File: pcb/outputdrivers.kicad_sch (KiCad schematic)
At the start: 24 parts, among them IC1 DRV8874QPWPRQ1, J7 CP/PE, J7 RF, Q1 BC846, Q2 NCV8402xST, Q3 NCV8402xST, Q4 DTA143Z, Q7 DTC114E, Q8 DTC114E, Q9 DTC114E, U7 74HCT04

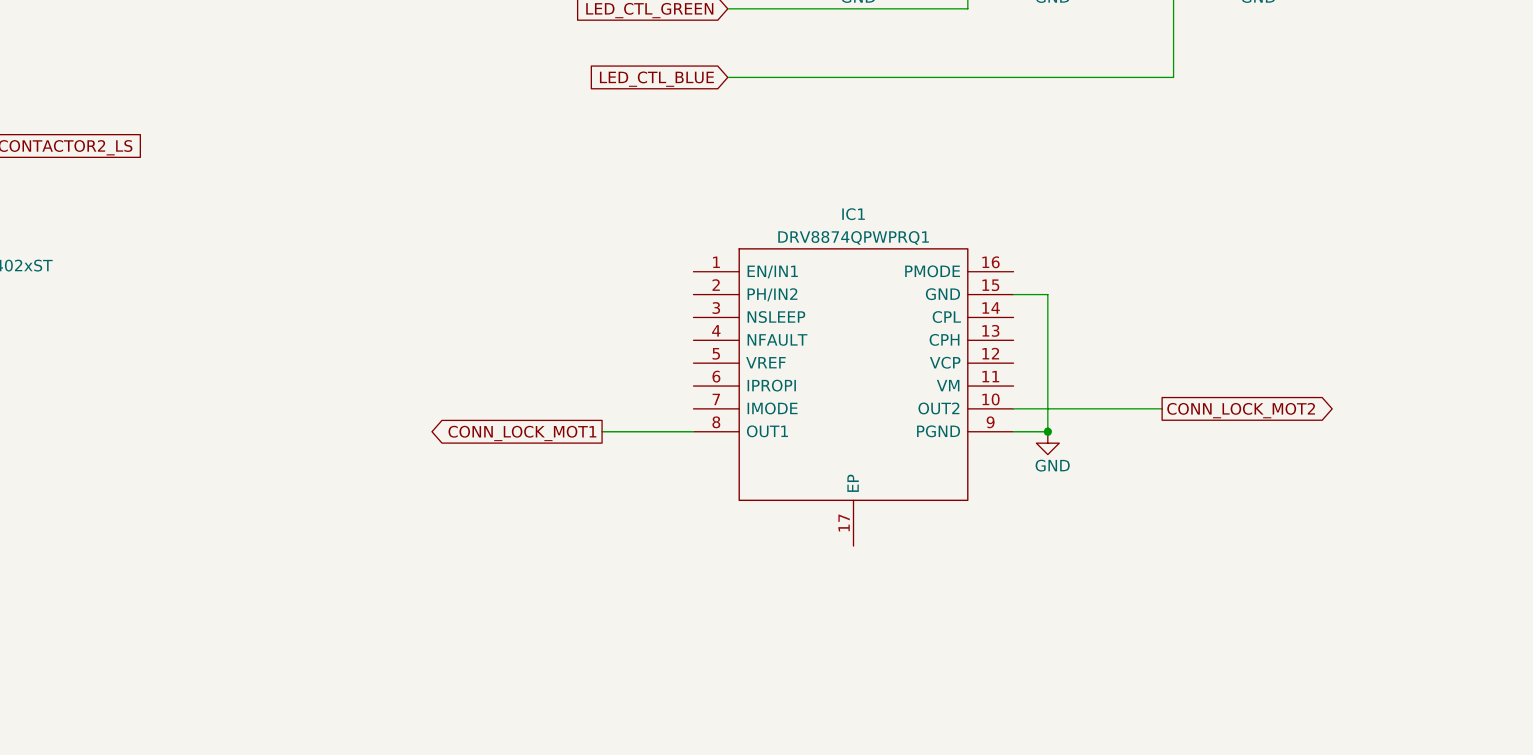
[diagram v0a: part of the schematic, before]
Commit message: wired the drv8874. Added spare holes. Flash connector larger holes
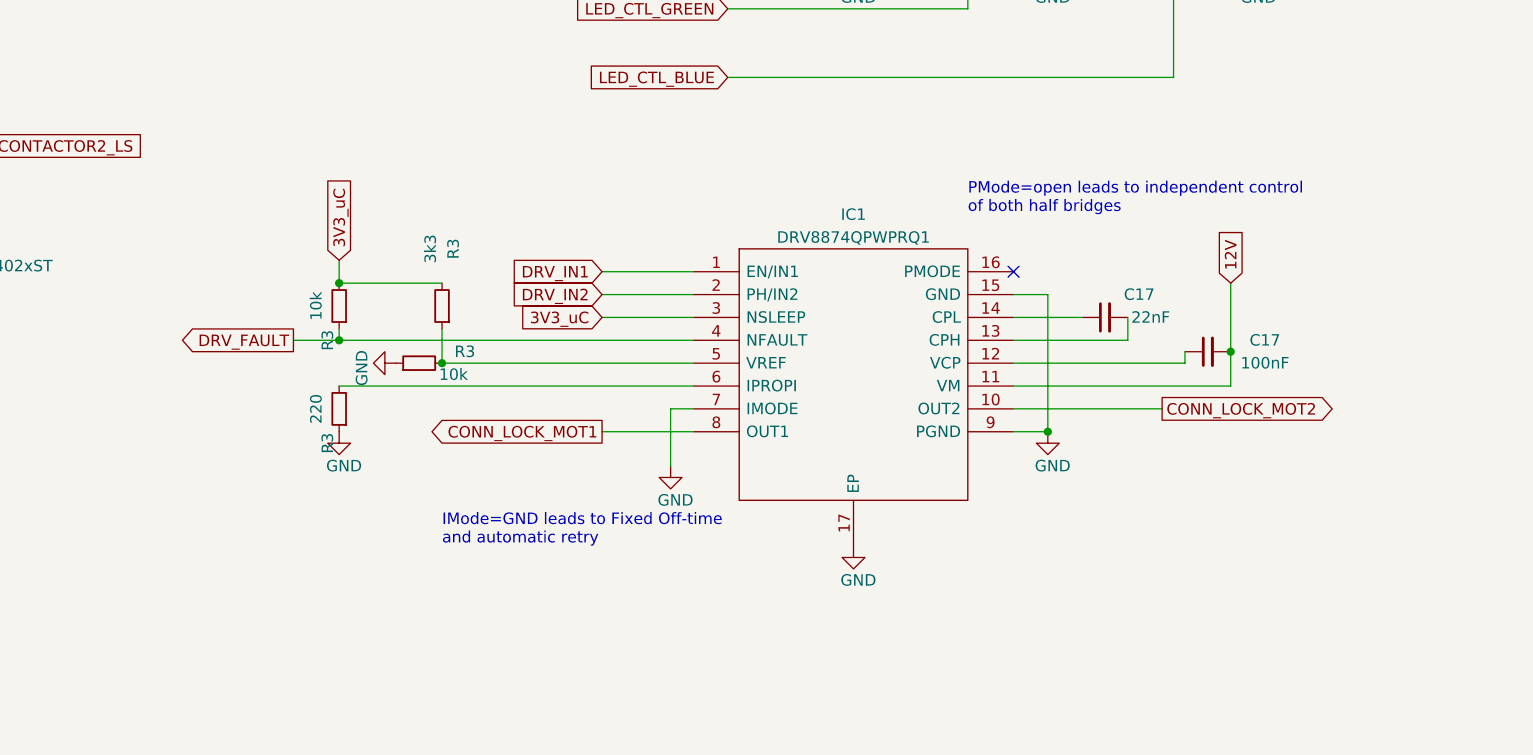
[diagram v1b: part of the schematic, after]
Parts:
- added C17: 100nF, Capacitor_SMD:C_0805_2012Metric_Pad1.18x1.45mm_HandSolder, symbol Device:C_Small
- added C17: 22nF, Capacitor_SMD:C_0805_2012Metric_Pad1.18x1.45mm_HandSolder, symbol Device:C_Small
- added R3: 3k3, Resistor_SMD:R_1206_3216Metric_Pad1.30x1.75mm_HandSolder, symbol Device:R_Small
- added R3: 220, Resistor_SMD:R_1206_3216Metric_Pad1.30x1.75mm_HandSolder, symbol Device:R_Small
- added R3 (x2): 10k, Resistor_SMD:R_1206_3216Metric_Pad1.30x1.75mm_HandSolder, symbol Device:R_Small
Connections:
- net GND: now also IC1.17 (EP), IC1.7 (IMODE), R3.1, R3.1
- net DRV_IN1: now reaches IC1.1 (EN/IN1)
- net 12V: now reaches IC1.11 (VM)
- net 12V: now also C17.2
- net at IC1.12 (VCP): now also C17.1
- net at IC1.13 (CPH): now also C17.2
- net at IC1.14 (CPL): now also C17.1
- net DRV_IN2: now reaches IC1.2 (PH/IN2)
- net 3V3_uC: now reaches IC1.3 (NSLEEP)
- net 3V3_uC: now also R3.2, R3.2
- net DRV_FAULT: now reaches IC1.4 (NFAULT)
- net DRV_FAULT: now also R3.1
- net at IC1.5 (VREF): now also R3.1, R3.2
- net at IC1.6 (IPROPI): now also R3.2
- no-connect marks 2 -> 3
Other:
- note added: "IMode=GND leads to Fixed Off-time and automatic retry"
- note added: "PMode=open leads to independent control of both half bridges"
